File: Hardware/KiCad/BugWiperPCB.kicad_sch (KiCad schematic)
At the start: 12 parts, among them J2 1770924, J3 Phoenix_1776508, J6 1824420000

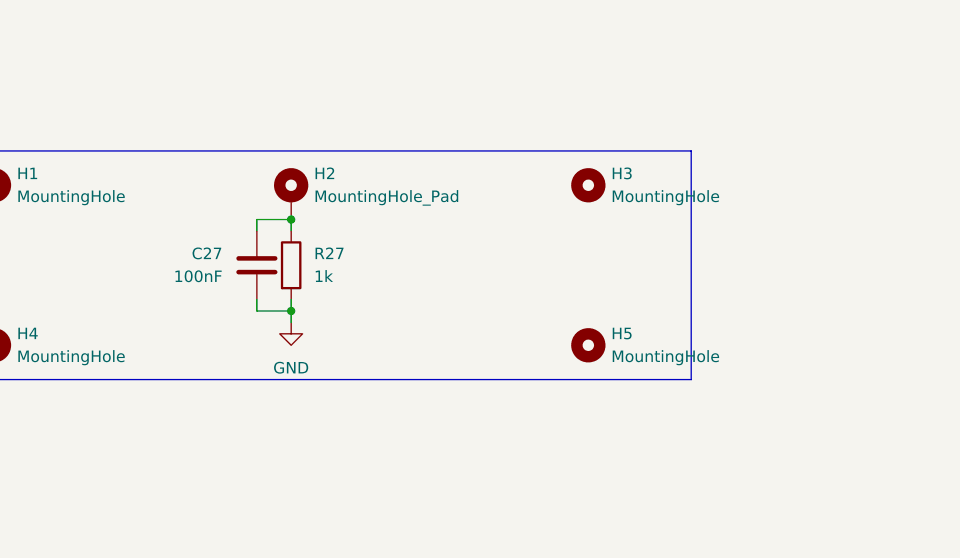
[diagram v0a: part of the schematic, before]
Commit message: update PCB
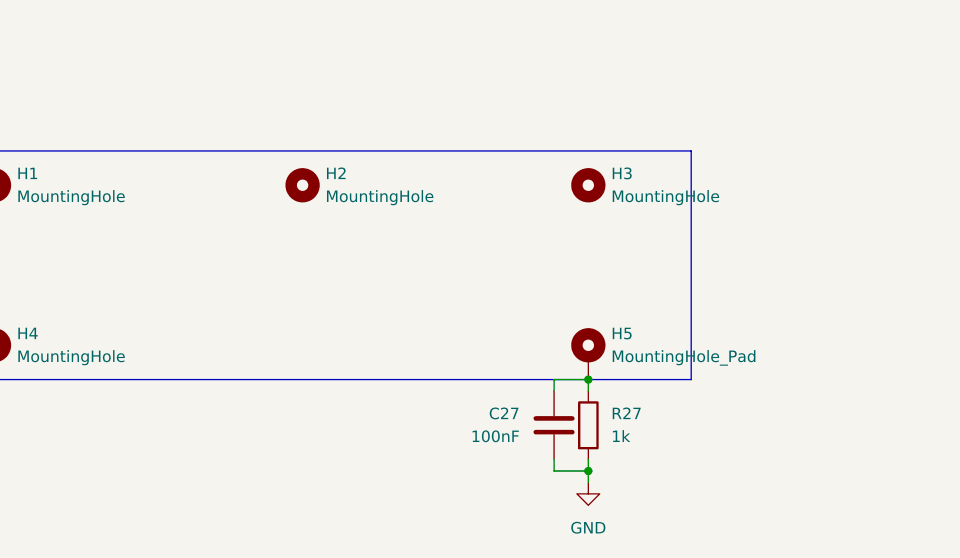
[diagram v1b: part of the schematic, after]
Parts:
- renumbered H5 to H2, H2 to H5
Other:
- moved on the sheet: C27, H2, H5, R27
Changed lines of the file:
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@@
 (kicad_sch (version 20230121) (generator eeschema)
   (paper "A4")
-  (junction (at 81.28 158.75) (diameter 0) (color 0 0 0 0)
-  )
-  (junction (at 81.28 148.59) (diameter 0) (color 0 0 0 0)
+  (junction (at 114.3 176.53) (diameter 0) (color 0 0 0 0)
+  )
+  (junction (at 114.3 166.37) (diameter 0) (color 0 0 0 0)
   )
   (junction (at 255.27 151.13) (diameter 0) (color 0 0 0 0)
@@
     (stroke (width 0) (type default))
   )
-  (wire (pts (xy 77.47 158.75) (xy 77.47 157.48))
+  (wire (pts (xy 110.49 176.53) (xy 110.49 175.26))
     (stroke (width 0) (type default))
   )
@@
     (stroke (width 0) (type default))
   )
-  (wire (pts (xy 81.28 158.75) (xy 81.28 160.02))
+  (wire (pts (xy 114.3 176.53) (xy 114.3 177.8))
     (stroke (width 0) (type default))
   )
@@
     (stroke (width 0) (type default))
   )
-  (wire (pts (xy 77.47 148.59) (xy 81.28 148.59))
+  (wire (pts (xy 110.49 166.37) (xy 114.3 166.37))
     (stroke (width 0) (type default))
   )
@@
     (stroke (width 0) (type default))
   )
-  (wire (pts (xy 81.28 158.75) (xy 81.28 157.48))
-    (stroke (width 0) (type default))
-  )
-  (wire (pts (xy 77.47 158.75) (xy 81.28 158.75))
+  (wire (pts (xy 114.3 176.53) (xy 114.3 175.26))
+    (stroke (width 0) (type default))
+  )
+  (wire (pts (xy 110.49 176.53) (xy 114.3 176.53))
     (stroke (width 0) (type default))
   )
@@
     (stroke (width 0) (type default))
   )
-  (wire (pts (xy 81.28 148.59) (xy 81.28 149.86))
-    (stroke (width 0) (type default))
-  )
-  (wire (pts (xy 77.47 148.59) (xy 77.47 149.86))
+  (wire (pts (xy 114.3 166.37) (xy 114.3 167.64))
+    (stroke (width 0) (type default))
+  )
+  (wire (pts (xy 110.49 166.37) (xy 110.49 167.64))
     (stroke (width 0) (type default))
   )
@@
     )
   )
-  (symbol (lib_id "Device:C") (at 77.47 153.67 0) (mirror y) (unit 1)
+  (symbol (lib_id "Device:C") (at 110.49 171.45 0) (mirror y) (unit 1)
     (in_bom yes) (on_board yes) (dnp no)
-    (property "Reference" "C27" (at 73.66 152.4 0)
-      (effects (font (size 1.27 1.27)) (justify left))
-    )
-    (property "Value" "100nF" (at 73.66 154.94 0)
-      (effects (font (size 1.27 1.27)) (justify left))
-    )
-    (property "Footprint" "Capacitor_SMD:C_0603_1608Metric" (at 76.5048 157.48 0)
-      (effects (font (size 1.27 1.27)) hide)
-    )
-    (property "Datasheet" "~" (at 77.47 153.67 0)
+    (property "Reference" "C27" (at 106.68 170.18 0)
+      (effects (font (size 1.27 1.27)) (justify left))
+    )
+    (property "Value" "100nF" (at 106.68 172.72 0)
+      (effects (font (size 1.27 1.27)) (justify left))
+    )
+    (property "Footprint" "Capacitor_SMD:C_0603_1608Metric" (at 109.5248 175.26 0)
+      (effects (font (size 1.27 1.27)) hide)
+    )
+    (property "Datasheet" "~" (at 110.49 171.45 0)
       (effects (font (size 1.27 1.27)) hide)
     )
@@
     )
   )
-  (symbol (lib_id "Mechanical:MountingHole_Pad") (at 81.28 146.05 0) (unit 1)
-    (in_bom yes) (on_board yes) (dnp no) (fields_autoplaced)
-    (property "Reference" "H2" (at 83.82 143.51 0)
-      (effects (font (size 1.27 1.27)) (justify left))
-    )
-    (property "Value" "MountingHole_Pad" (at 83.82 146.05 0)
-      (effects (font (size 1.27 1.27)) (justify left))
-    )
-    (property "Footprint" "MountingHole:MountingHole_3.2mm_M3_DIN965_Pad_TopBottom" (at 81.28 146.05 0)
-      (effects (font (size 1.27 1.27)) hide)
-    )
-    (property "Datasheet" "~" (at 81.28 146.05 0)
-      (effects (font (size 1.27 1.27)) hide)
-    )
-    (pin "1")
+  (symbol (lib_id "Mechanical:MountingHole_Pad") (at 114.3 163.83 0) (unit 1)
+    (in_bom yes) (on_board yes) (dnp no) (fields_autoplaced)
+    (property "Reference" "H5" (at 116.84 161.29 0)
+      (effects (font (size 1.27 1.27)) (justify left))
+    )
+    (property "Value" "MountingHole_Pad" (at 116.84 163.83 0)
+      (effects (font (size 1.27 1.27)) (justify left))
+    )
+    (property "Footprint" "MountingHole:MountingHole_3.2mm_M3_DIN965_Pad_TopBottom" (at 114.3 163.83 0)
+      (effects (font (size 1.27 1.27)) hide)
+    )
+    (property "Datasheet" "~" (at 114.3 163.83 0)
+      (effects (font (size 1.27 1.27)) hide)
+    )
+    (pin "1")
+    (instances
+      (project "BugWiperPCB"
+        (path "/d31a15bd-db02-4d4c-9593-17c596d3182c"
+          (reference "H5") (unit 1)
+        )
+      )
+    )
+  )
+  (symbol (lib_id "power:GND") (at 114.3 177.8 0) (unit 1)
+    (in_bom yes) (on_board yes) (dnp no) (fields_autoplaced)
+    (property "Reference" "#PWR034" (at 114.3 184.15 0)
+      (effects (font (size 1.27 1.27)) hide)
+    )
+    (property "Value" "GND" (at 114.3 182.88 0)
+      (effects (font (size 1.27 1.27)))
+    )
+    (property "Footprint" "" (at 114.3 177.8 0)
+      (effects (font (size 1.27 1.27)) hide)
+    )
+    (property "Datasheet" "" (at 114.3 177.8 0)
+      (effects (font (size 1.27 1.27)) hide)
+    )
+    (pin "1")
+    (instances
+      (project "BugWiperPCB"
+        (path "/d31a15bd-db02-4d4c-9593-17c596d3182c"
+          (reference "#PWR034") (unit 1)
+        )
+      )
+    )
+  )
+  (symbol (lib_id "Mechanical:MountingHole") (at 82.55 144.78 0) (unit 1)
+    (in_bom yes) (on_board yes) (dnp no) (fields_autoplaced)
+    (property "Reference" "H2" (at 85.09 143.51 0)
+      (effects (font (size 1.27 1.27)) (justify left))
+    )
+    (property "Value" "MountingHole" (at 85.09 146.05 0)
+      (effects (font (size 1.27 1.27)) (justify left))
+    )
+    (property "Footprint" "MountingHole:MountingHole_3.2mm_M3_DIN965" (at 82.55 144.78 0)
+      (effects (font (size 1.27 1.27)) hide)
+    )
+    (property "Datasheet" "~" (at 82.55 144.78 0)
+      (effects (font (size 1.27 1.27)) hide)
+    )
     (instances
       (project "BugWiperPCB"
@@
     )
   )
-  (symbol (lib_id "power:GND") (at 81.28 160.02 0) (unit 1)
-    (in_bom yes) (on_board yes) (dnp no) (fields_autoplaced)
-    (property "Reference" "#PWR034" (at 81.28 166.37 0)
-      (effects (font (size 1.27 1.27)) hide)
-    )
-    (property "Value" "GND" (at 81.28 165.1 0)
-      (effects (font (size 1.27 1.27)))
-    )
-    (property "Footprint" "" (at 81.28 160.02 0)
-      (effects (font (size 1.27 1.27)) hide)
-    )
-    (property "Datasheet" "" (at 81.28 160.02 0)
-      (effects (font (size 1.27 1.27)) hide)
-    )
-    (pin "1")
-    (instances
-      (project "BugWiperPCB"
-        (path "/d31a15bd-db02-4d4c-9593-17c596d3182c"
-          (reference "#PWR034") (unit 1)
-        )
-      )
-    )
-  )
-  (symbol (lib_id "Mechanical:MountingHole") (at 114.3 162.56 0) (unit 1)
-    (in_bom yes) (on_board yes) (dnp no) (fields_autoplaced)
-    (property "Reference" "H5" (at 116.84 161.29 0)
-      (effects (font (size 1.27 1.27)) (justify left))
-    )
-    (property "Value" "MountingHole" (at 116.84 163.83 0)
-      (effects (font (size 1.27 1.27)) (justify left))
-    )
-    (property "Footprint" "MountingHole:MountingHole_3.2mm_M3_DIN965" (at 114.3 162.56 0)
-      (effects (font (size 1.27 1.27)) hide)
-    )
-    (property "Datasheet" "~" (at 114.3 162.56 0)
-      (effects (font (size 1.27 1.27)) hide)
-    )
-    (instances
-      (project "BugWiperPCB"
-        (path "/d31a15bd-db02-4d4c-9593-17c596d3182c"
-          (reference "H5") (unit 1)
-        )
-      )
-    )
-  )
-  (symbol (lib_id "Device:R") (at 81.28 153.67 0) (unit 1)
-    (in_bom yes) (on_board yes) (dnp no) (fields_autoplaced)
-    (property "Reference" "R27" (at 83.82 152.4 0)
-      (effects (font (size 1.27 1.27)) (justify left))
-    )
-    (property "Value" "1k" (at 83.82 154.94 0)
-      (effects (font (size 1.27 1.27)) (justify left))
-    )
-    (property "Footprint" "Resistor_SMD:R_0603_1608Metric" (at 79.502 153.67 90)
-      (effects (font (size 1.27 1.27)) hide)
-    )
-    (property "Datasheet" "~" (at 81.28 153.67 0)
-      (effects (font (size 1.27 1.27)) hide)
-    )
+  (symbol (lib_id "Device:R") (at 114.3 171.45 0) (unit 1)
+    (in_bom yes) (on_board yes) (dnp no) (fields_autoplaced)
+    (property "Reference" "R27" (at 116.84 170.18 0)
+      (effects (font (size 1.27 1.27)) (justify left))
+    )
+    (property "Value" "1k" (at 116.84 172.72 0)
+      (effects (font (size 1.27 1.27)) (justify left))
+    )
+    (property "Footprint" "Resistor_SMD:R_0603_1608Metric" (at 112.522 171.45 90)
+      (effects (font (size 1.27 1.27)) hide)
+    )
+    (property "Datasheet" "~" (at 114.3 171.45 0)
+      (effects (font (size 1.27 1.27)) hide)
+    )
